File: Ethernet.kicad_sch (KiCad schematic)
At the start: 23 parts, among them J13 RJ45_Halo_HFJ11-x2450E-LxxRL, U9 LAN8720A

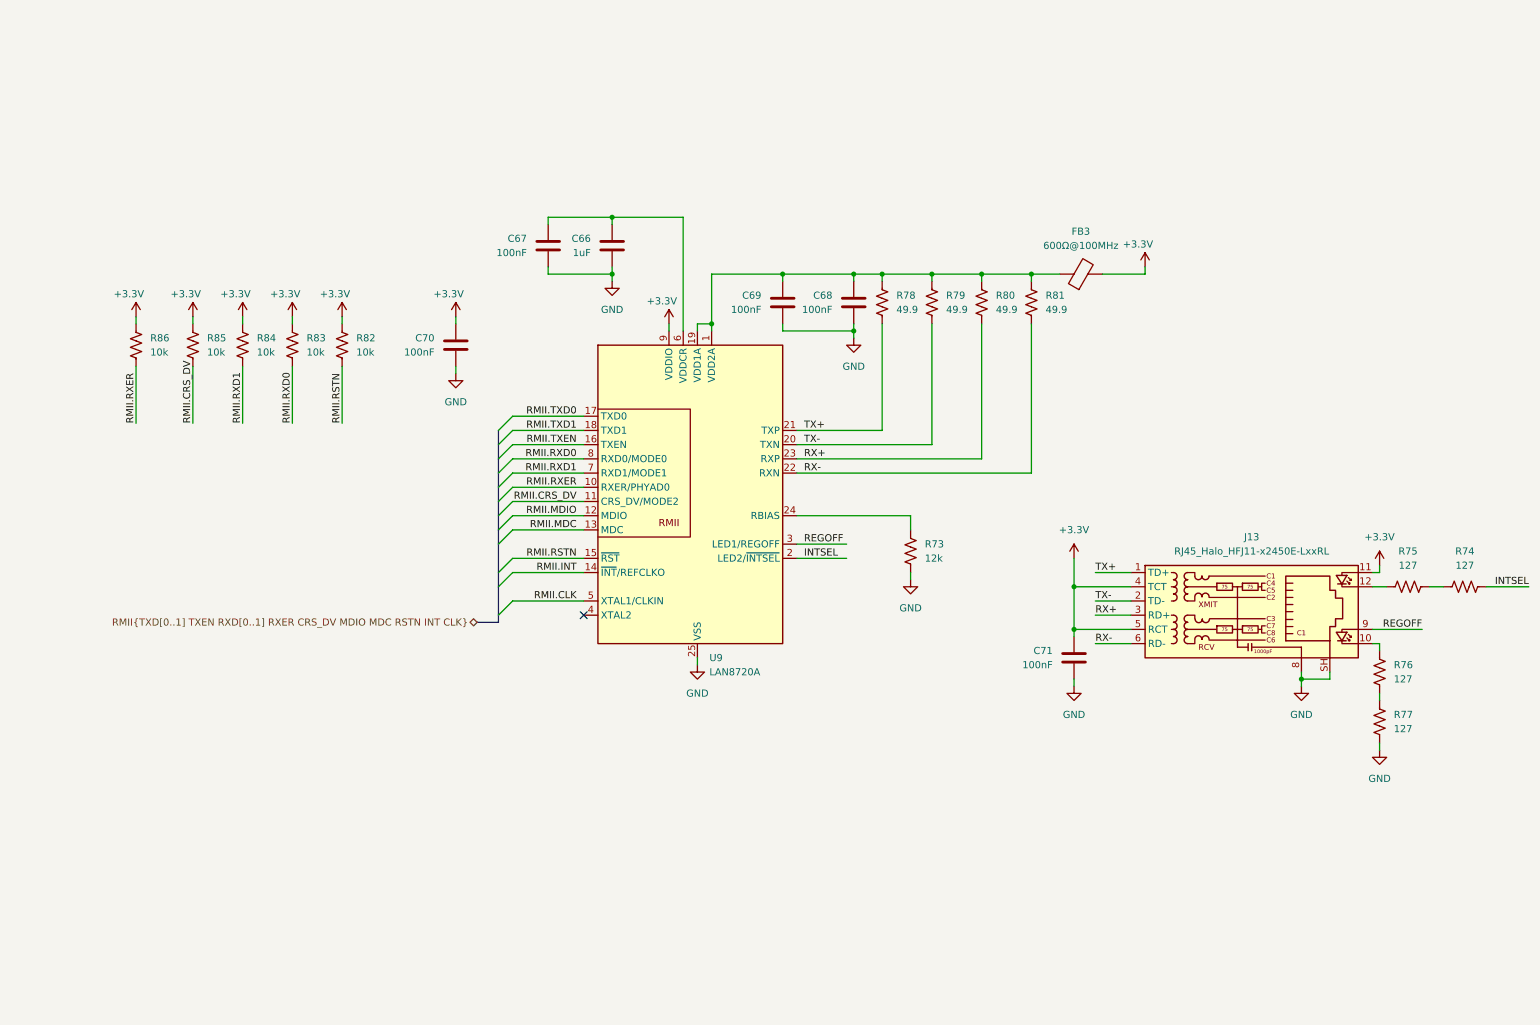
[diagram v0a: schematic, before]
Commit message: Cleanup
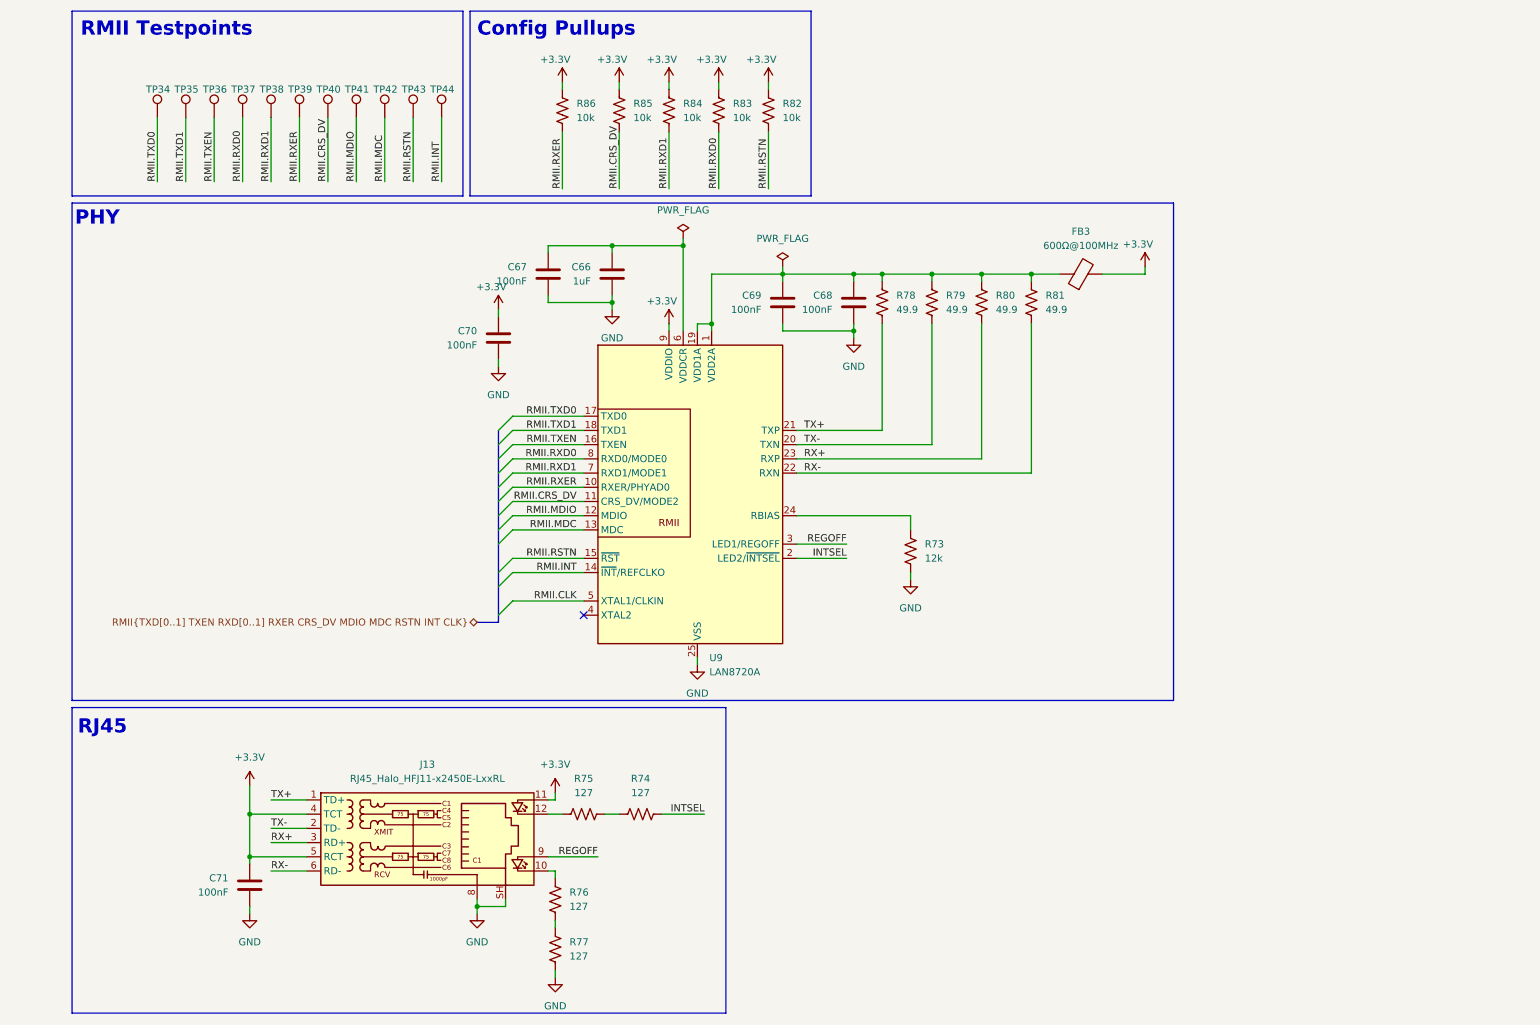
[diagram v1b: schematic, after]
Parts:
- added TP34, TP35, TP36, TP37, TP38, TP39, TP40, TP41, TP42, TP43, TP44: TestPoint, TestPoint:TestPoint_Pad_D2.0mm, symbol Connector:TestPoint
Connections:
- net RMII.CRS_DV: now also TP40.1
- net RMII.INT: now also TP44.1
- net RMII.MDC: now also TP42.1
- net RMII.MDIO: now also TP41.1
- net RMII.RSTN: now also TP43.1
- net RMII.RXD0: now also TP37.1
- net RMII.RXD1: now also TP38.1
- net RMII.RXER: now also TP39.1
- net RMII.TXD0: now also TP34.1
- net RMII.TXD1: now also TP35.1
- net RMII.TXEN: now also TP36.1
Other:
- note added: "Config Pullups"
- note added: "PHY"
- note added: "RJ45"
- note added: "RMII Testpoints"
- title: (none) -> Ethernet
- moved on the sheet: C66, C67, C70, C71, J13, R74, R75, R76, R77, R82, R83, R84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
